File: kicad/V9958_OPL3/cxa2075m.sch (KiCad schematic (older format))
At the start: 33 parts, among them P1 RED, P2 GREEN, P3 BLUE, P4 SYNC/C, U7 cxa2075M, X1 OSC, X3 S-VIDEO

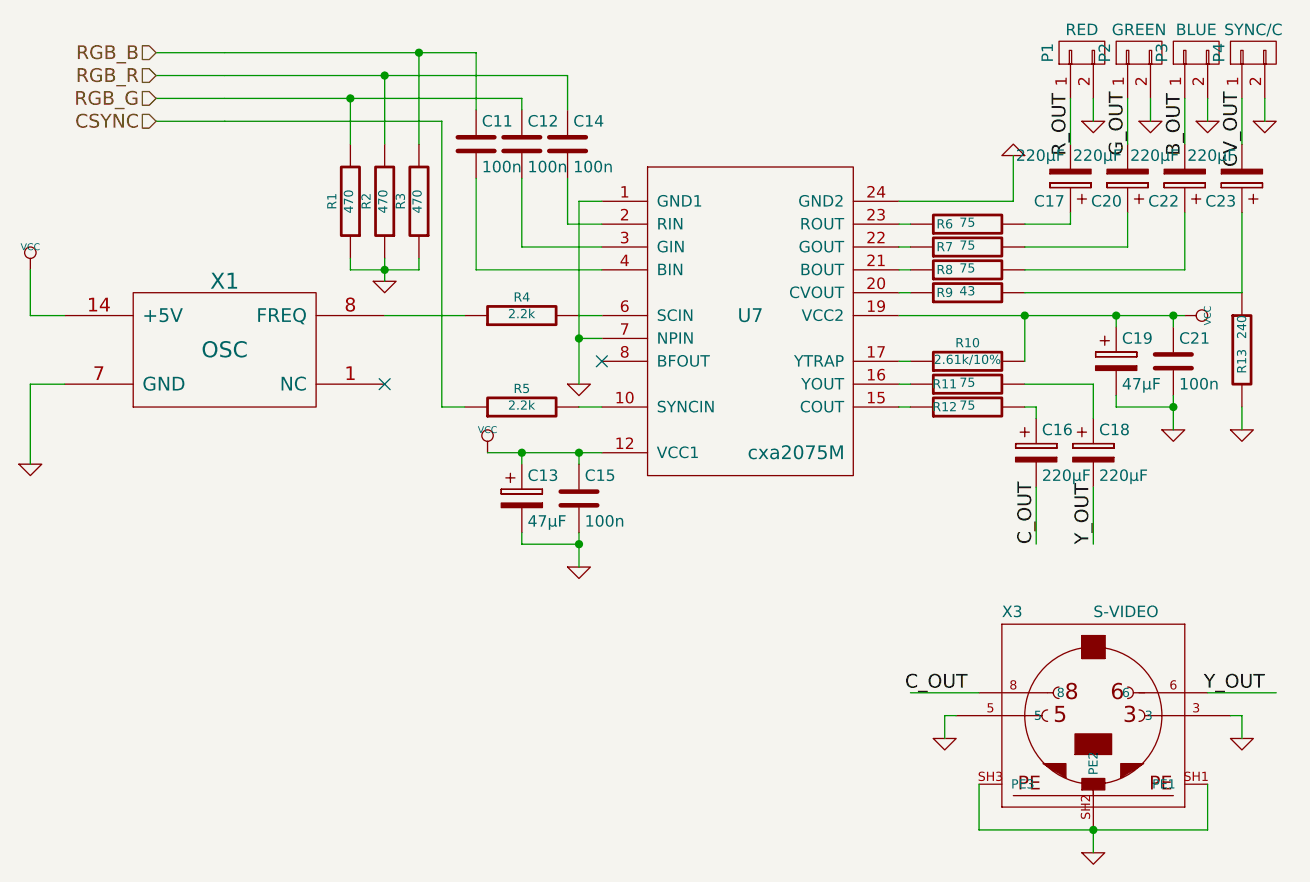
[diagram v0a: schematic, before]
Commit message: update
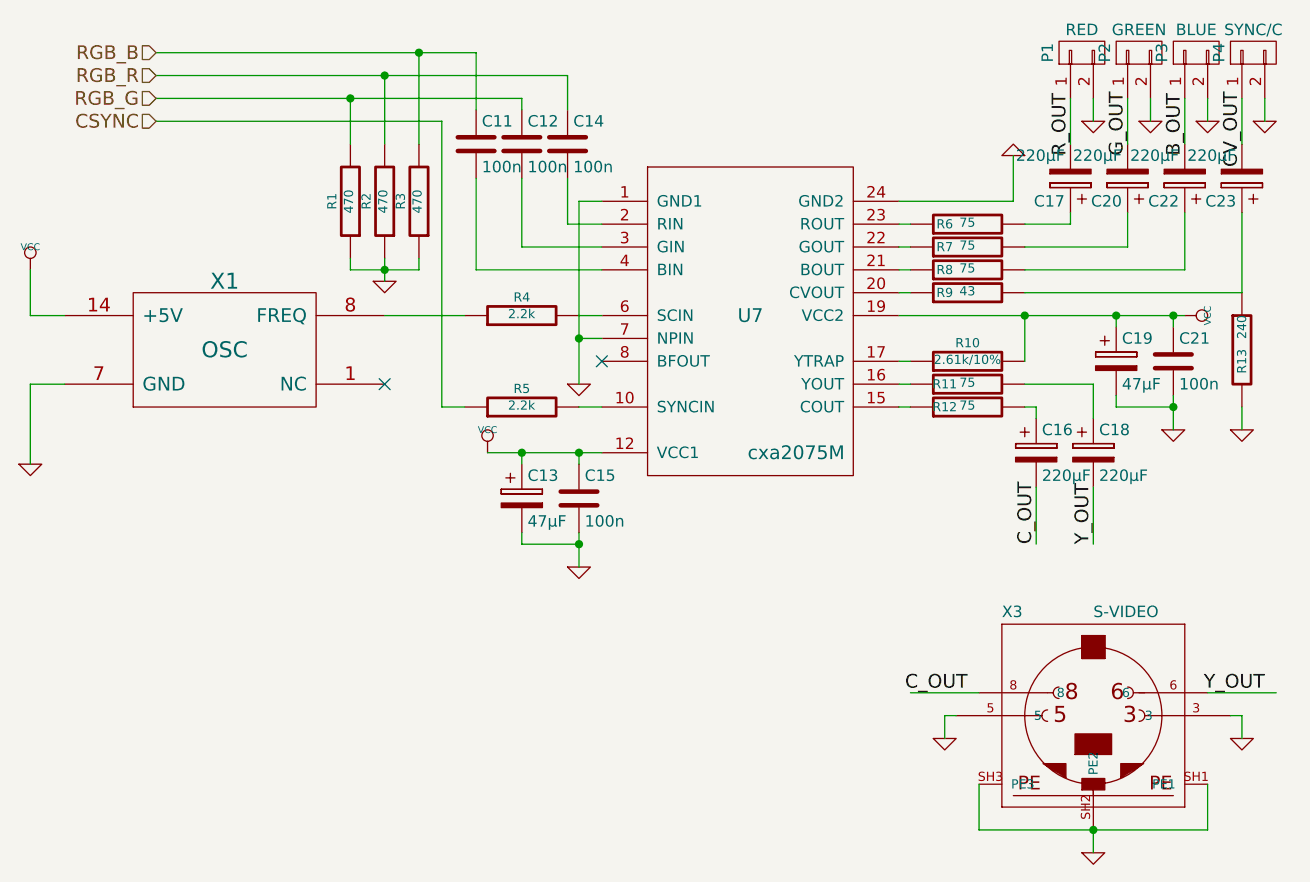
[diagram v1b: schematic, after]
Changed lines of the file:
@@
 $EndComp
 $Comp
-L GND-RESCUE-v9958 #PWR27
+L GND-RESCUE-v9958 #PWR025
 U 1 1 5B035F00
 P 4450 3850
-F 0 "#PWR27" H 4450 3850 30  0001 C CNN
+F 0 "#PWR025" H 4450 3850 30  0001 C CNN
 F 1 "GND" H 4450 3780 30  0001 C CNN
 F 2 "" H 4450 3850 60  0000 C CNN
@@
 $EndComp
 $Comp
-L GND-RESCUE-v9958 #PWR29
+L GND-RESCUE-v9958 #PWR026
 U 1 1 5B035F0D
 P 5300 4300
-F 0 "#PWR29" H 5300 4300 30  0001 C CNN
+F 0 "#PWR026" H 5300 4300 30  0001 C CNN
 F 1 "GND" H 5300 4230 30  0001 C CNN
 F 2 "" H 5300 4300 60  0000 C CNN
@@
 $EndComp
 $Comp
-L GND-RESCUE-v9958 #PWR32
+L GND-RESCUE-v9958 #PWR027
 U 1 1 5B035F13
 P 7200 3300
-F 0 "#PWR32" H 7200 3300 30  0001 C CNN
+F 0 "#PWR027" H 7200 3300 30  0001 C CNN
 F 1 "GND" H 7200 3230 30  0001 C CNN
 F 2 "" H 7200 3300 60  0000 C CNN
@@
 $EndComp
 $Comp
-L VCC #PWR28
+L VCC #PWR028
 U 1 1 5B035F19
 P 4900 4600
-F 0 "#PWR28" H 4900 4700 30  0001 C CNN
+F 0 "#PWR028" H 4900 4700 30  0001 C CNN
 F 1 "VCC" H 4900 4700 30  0000 C CNN
 F 2 "" H 4900 4600 60  0000 C CNN
@@
 $EndComp
 $Comp
-L VCC #PWR37
+L VCC #PWR029
 U 1 1 5B035F1F
 P 7950 4000
-F 0 "#PWR37" H 7950 4100 30  0001 C CNN
+F 0 "#PWR029" H 7950 4100 30  0001 C CNN
 F 1 "VCC" H 7950 4100 30  0000 C CNN
 F 2 "" H 7950 4000 60  0000 C CNN
@@
 $EndComp
 $Comp
-L GND-RESCUE-v9958 #PWR39
+L GND-RESCUE-v9958 #PWR030
 U 1 1 5B035F87
 P 8200 4500
-F 0 "#PWR39" H 8200 4500 30  0001 C CNN
+F 0 "#PWR030" H 8200 4500 30  0001 C CNN
 F 1 "GND" H 8200 4430 30  0001 C CNN
 F 2 "" H 8200 4500 60  0000 C CNN
@@
 $EndComp
 $Comp
-L GND-RESCUE-v9958 #PWR30
+L GND-RESCUE-v9958 #PWR031
 U 1 1 5B035FB7
 P 5300 5100
-F 0 "#PWR30" H 5300 5100 30  0001 C CNN
+F 0 "#PWR031" H 5300 5100 30  0001 C CNN
 F 1 "GND" H 5300 5030 30  0001 C CNN
 F 2 "" H 5300 5100 60  0000 C CNN
@@
 $EndComp
 $Comp
-L GND-RESCUE-v9958 #PWR36
+L GND-RESCUE-v9958 #PWR032
 U 1 1 5B035FCB
 P 7900 4500
-F 0 "#PWR36" H 7900 4500 30  0001 C CNN
+F 0 "#PWR032" H 7900 4500 30  0001 C CNN
 F 1 "GND" H 7900 4430 30  0001 C CNN
 F 2 "" H 7900 4500 60  0000 C CNN
@@
 $EndComp
 $Comp
-L VCC #PWR25
+L VCC #PWR033
 U 1 1 5B035FD8
 P 2900 3800
-F 0 "#PWR25" H 2900 3900 30  0001 C CNN
+F 0 "#PWR033" H 2900 3900 30  0001 C CNN
 F 1 "VCC" H 2900 3900 30  0000 C CNN
 F 2 "" H 2900 3800 60  0000 C CNN
@@
 $EndComp
 $Comp
-L GND-RESCUE-v9958 #PWR26
+L GND-RESCUE-v9958 #PWR034
 U 1 1 5B035FDE
 P 2900 4650
-F 0 "#PWR26" H 2900 4650 30  0001 C CNN
+F 0 "#PWR034" H 2900 4650 30  0001 C CNN
 F 1 "GND" H 2900 4580 30  0001 C CNN
 F 2 "" H 2900 4650 60  0000 C CNN
@@
 $EndComp
 $Comp
-L GND-RESCUE-v9958 #PWR33
+L GND-RESCUE-v9958 #PWR035
 U 1 1 5B03600E
 P 7550 3150
-F 0 "#PWR33" H 7550 3150 30  0001 C CNN
+F 0 "#PWR035" H 7550 3150 30  0001 C CNN
 F 1 "GND" H 7550 3080 30  0001 C CNN
 F 2 "" H 7550 3150 60  0000 C CNN
@@
 $EndComp
 $Comp
-L GND-RESCUE-v9958 #PWR35
+L GND-RESCUE-v9958 #PWR036
 U 1 1 5B036014
 P 7800 3150
-F 0 "#PWR35" H 7800 3150 30  0001 C CNN
+F 0 "#PWR036" H 7800 3150 30  0001 C CNN
 F 1 "GND" H 7800 3080 30  0001 C CNN
 F 2 "" H 7800 3150 60  0000 C CNN
@@
 $EndComp
 $Comp
-L GND-RESCUE-v9958 #PWR38
+L GND-RESCUE-v9958 #PWR037
 U 1 1 5B03601A
 P 8050 3150
-F 0 "#PWR38" H 8050 3150 30  0001 C CNN
+F 0 "#PWR037" H 8050 3150 30  0001 C CNN
 F 1 "GND" H 8050 3080 30  0001 C CNN
 F 2 "" H 8050 3150 60  0000 C CNN
@@
 $EndComp
 $Comp
-L GND-RESCUE-v9958 #PWR41
+L GND-RESCUE-v9958 #PWR038
 U 1 1 5B036020
 P 8300 3150
-F 0 "#PWR41" H 8300 3150 30  0001 C CNN
+F 0 "#PWR038" H 8300 3150 30  0001 C CNN
 F 1 "GND" H 8300 3080 30  0001 C CNN
 F 2 "" H 8300 3150 60  0000 C CNN
@@
 $EndComp
 Wire Wire Line
-	3750 3050 5050 3050
+	3450 3050 5050 3050
 Wire Wire Line
 	4300 3050 4300 3250
@@
 Connection ~ 4300 3050
 Wire Wire Line
-	3750 2950 5250 2950
+	3450 2950 5250 2950
 Connection ~ 4450 2950
 Wire Wire Line
-	3750 2850 4850 2850
+	3450 2850 4850 2850
 Connection ~ 4600 2850
 Wire Wire Line
 	5050 3050 5050 3100
 Wire Wire Line
-	3750 3150 4700 3150
+	3450 3150 4700 3150
 Wire Wire Line
 	4700 3150 4700 4400
@@
 Wire Wire Line
 	4850 2850 4850 3100
-Wire Wire Line
-	3450 2850 3750 2850
-Wire Wire Line
-	3450 2950 3750 2950
-Wire Wire Line
-	3450 3050 3750 3050
-Wire Wire Line
-	3450 3150 3750 3150
 Text HLabel 3450 2850 0    60   Input ~ 0
 RGB_B
@@
 $EndComp
 $Comp
-L GND-RESCUE-v9958 #PWR31
+L GND-RESCUE-v9958 #PWR039
 U 1 1 5B038CCB
 P 6900 5850
-F 0 "#PWR31" H 6900 5850 30  0001 C CNN
+F 0 "#PWR039" H 6900 5850 30  0001 C CNN
 F 1 "GND" H 6900 5780 30  0001 C CNN
 F 2 "" H 6900 5850 60  0000 C CNN
@@
 $EndComp
 $Comp
-L GND-RESCUE-v9958 #PWR40
+L GND-RESCUE-v9958 #PWR040
 U 1 1 5B038CD1
 P 8200 5850
-F 0 "#PWR40" H 8200 5850 30  0001 C CNN
+F 0 "#PWR040" H 8200 5850 30  0001 C CNN
 F 1 "GND" H 8200 5780 30  0001 C CNN
 F 2 "" H 8200 5850 60  0000 C CNN
@@
 	7050 6050 7050 6250
 Wire Wire Line
-	7050 6250 7550 6250
-Wire Wire Line
-	7550 6250 8050 6250
+	7050 6250 8050 6250
 Wire Wire Line
 	8050 6250 8050 6050
 Connection ~ 7550 6250
 $Comp
-L GND-RESCUE-v9958 #PWR34
+L GND-RESCUE-v9958 #PWR041
 U 1 1 5B038CE4
 P 7550 6350
-F 0 "#PWR34" H 7550 6350 30  0001 C CNN
+F 0 "#PWR041" H 7550 6350 30  0001 C CNN
 F 1 "GND" H 7550 6280 30  0001 C CNN
 F 2 "" H 7550 6350 60  0000 C CNN
